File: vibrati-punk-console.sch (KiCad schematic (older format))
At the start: 20 parts, among them U1 NE555, U2 NE555, U3 NE555

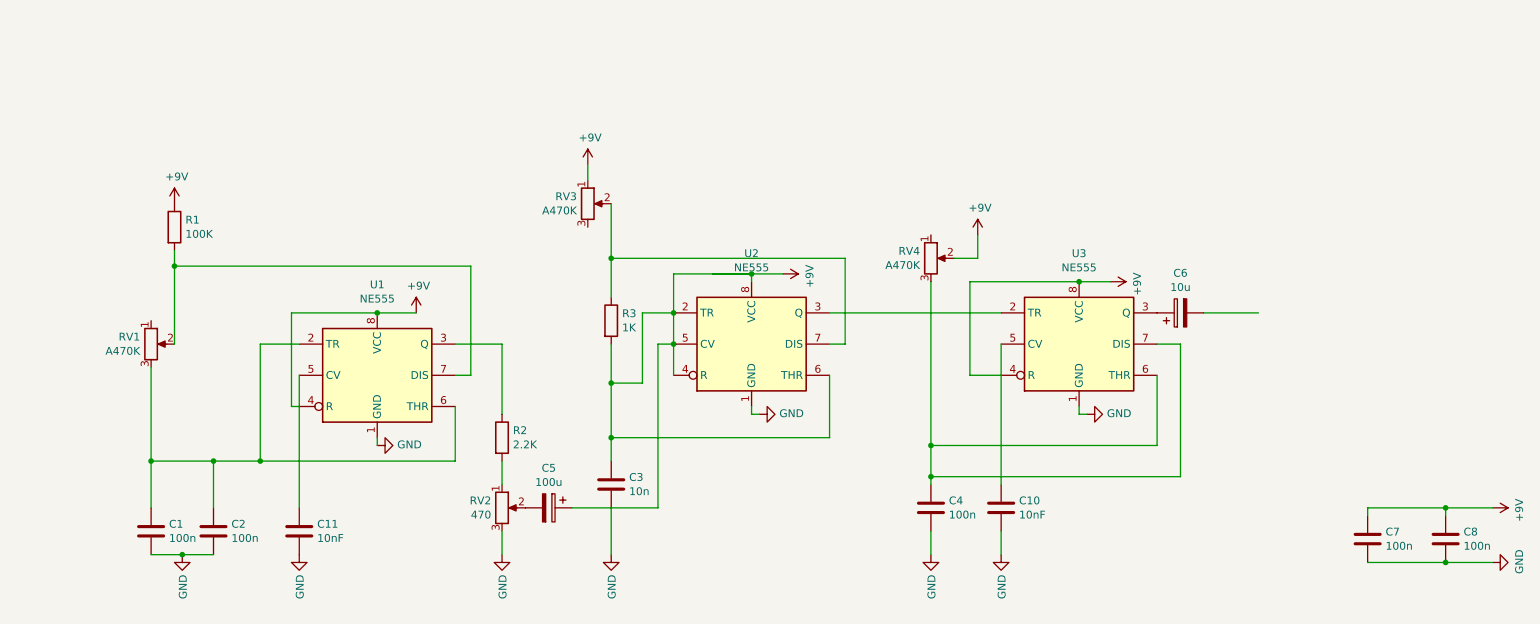
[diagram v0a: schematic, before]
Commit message: Further cleanup
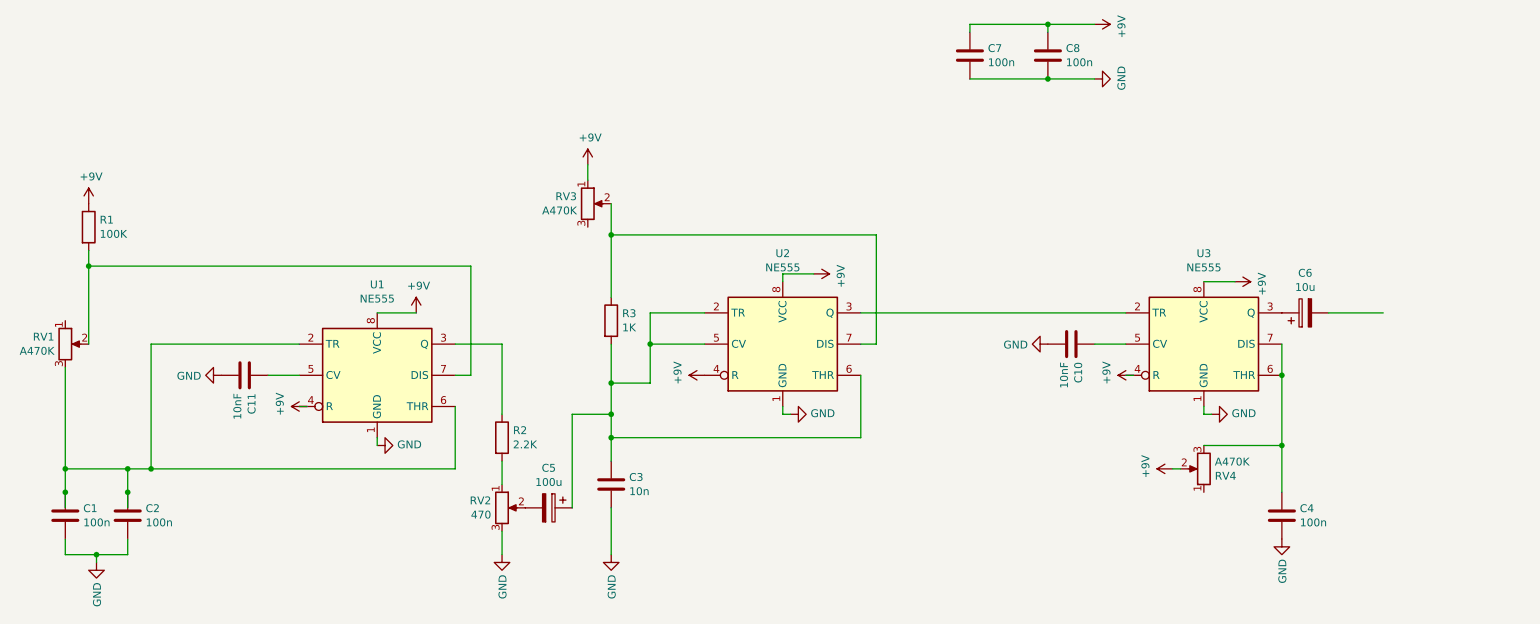
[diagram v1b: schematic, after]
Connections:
- wire segments 80 -> 71
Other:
- moved on the sheet: C1, C10, C11, C2, C4, C6, C7, C8, R1, RV1, RV4, U2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
